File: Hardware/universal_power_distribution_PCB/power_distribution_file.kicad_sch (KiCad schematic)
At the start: 87 parts, among them J1 Screw_Terminal_01x02, J10 Screw_Terminal_01x02, J2 Screw_Terminal_01x02, J3 Screw_Terminal_01x02, J4 Screw_Terminal_01x02, J5 Screw_Terminal_01x02, J6 Screw_Terminal_01x02, J7 Screw_Terminal_01x02, J8 Screw_Terminal_01x02, J9 Screw_Terminal_01x02, Q1 LMR51635XDDCR, Q2 LMR51635XDDCR, Q3 LMR51635XDDCR, Q4 LMR51635XDDCR, Q5 LMR51635XDDCR, Q6 BSS84, U1 INA228, U2 INA228, U3 ACS711xEXLT-31AB

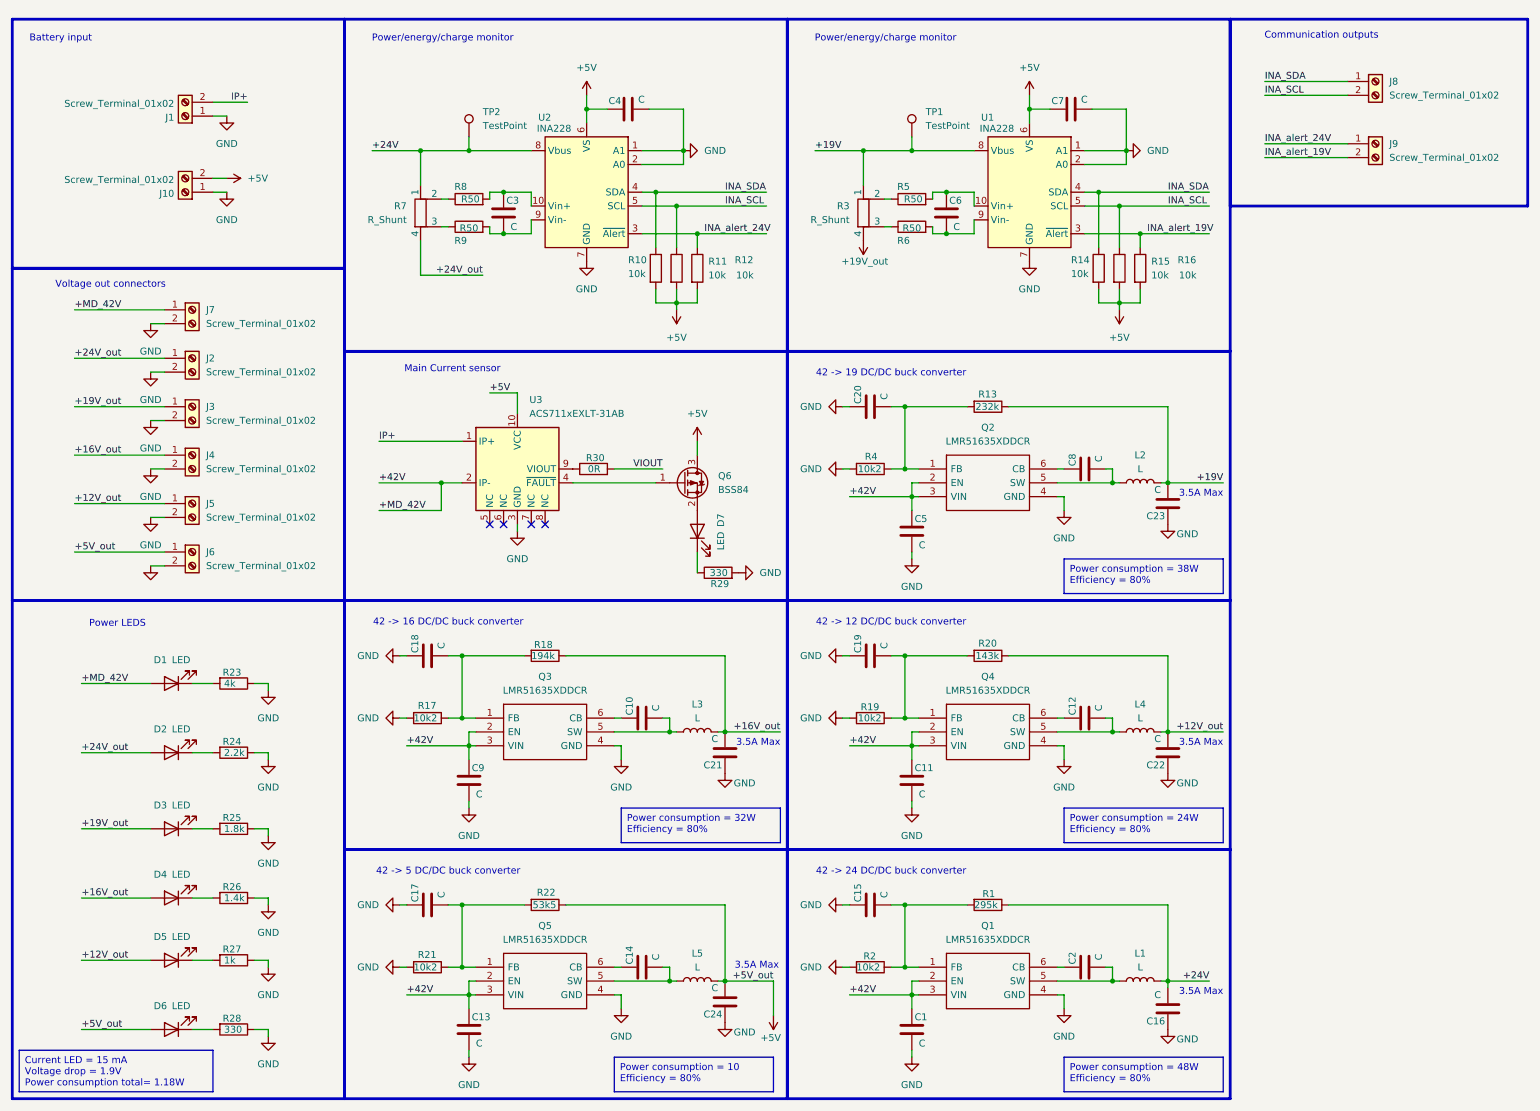
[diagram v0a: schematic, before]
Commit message: Restructured pcb
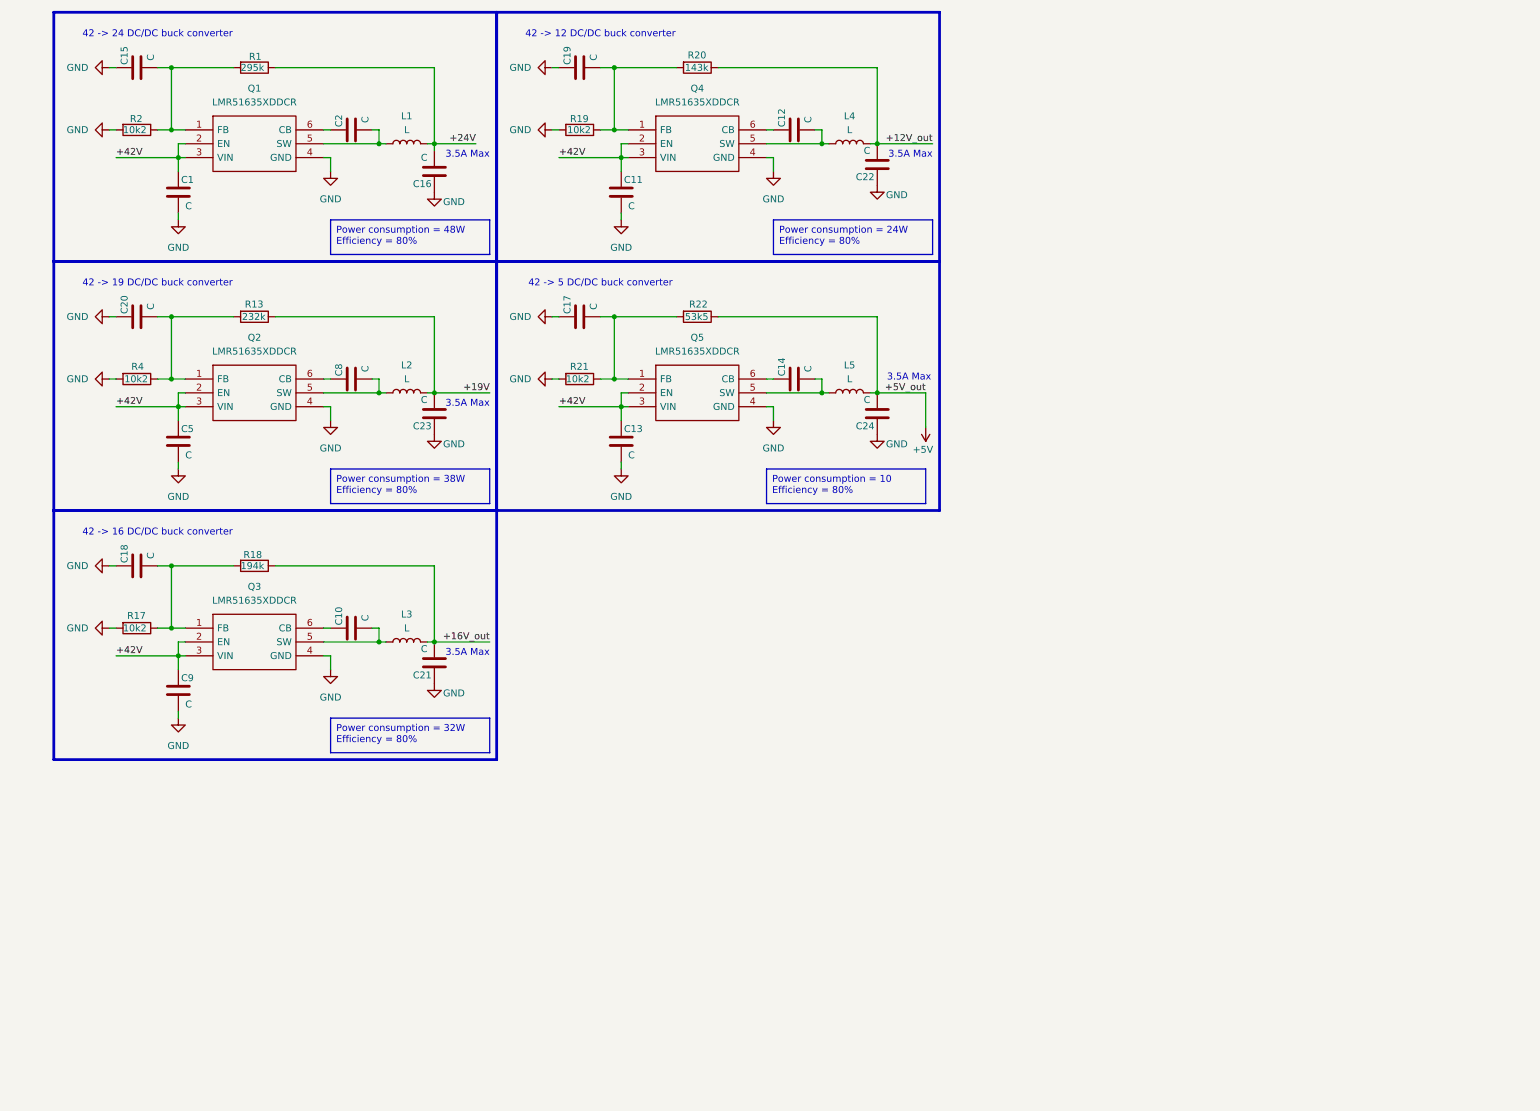
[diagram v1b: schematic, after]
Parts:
- removed C3, C4, C6, C7: C, symbol Device:C
- removed D1, D2, D3, D5, D6: LED, LED_SMD:LED_0603_1608Metric_Pad1.05x0.95mm_HandSolder, symbol Device:LED
- removed D4: LED, Resistor_SMD:R_0603_1608Metric_Pad0.98x0.95mm_HandSolder, symbol Device:LED
- removed D7: LED, symbol Device:LED
- removed J1, J10, J2, J3, J4, J5, J6, J7, J8, J9: Screw_Terminal_01x02, symbol Connector:Screw_Terminal_01x02
- removed Q6: BSS84, Package_TO_SOT_SMD:SOT-23, symbol Transistor_FET:BSS84
- removed R10, R11, R12, R14, R15, R16: 10k, Resistor_SMD:R_0603_1608Metric_Pad0.98x0.95mm_HandSolder, symbol Device:R
- removed R23: 4k, Resistor_SMD:R_0603_1608Metric_Pad0.98x0.95mm_HandSolder, symbol Device:R
- removed R24: 2.2k, Resistor_SMD:R_0603_1608Metric_Pad0.98x0.95mm_HandSolder, symbol Device:R
- removed R25: 1.8k, Resistor_SMD:R_0603_1608Metric_Pad0.98x0.95mm_HandSolder, symbol Device:R
- removed R26: 1.4k, Resistor_SMD:R_0603_1608Metric_Pad0.98x0.95mm_HandSolder, symbol Device:R
- removed R27: 1k, Resistor_SMD:R_0603_1608Metric_Pad0.98x0.95mm_HandSolder, symbol Device:R
- removed R28, R29: 330, Resistor_SMD:R_0603_1608Metric_Pad0.98x0.95mm_HandSolder, symbol Device:R
- removed R3, R7: R_Shunt, symbol Device:R_Shunt
- removed R30: 0R, Resistor_SMD:R_0603_1608Metric_Pad0.98x0.95mm_HandSolder, symbol Device:R
- removed R5, R6, R8, R9: R50, Resistor_SMD:R_0603_1608Metric_Pad0.98x0.95mm_HandSolder, symbol Device:R
- removed TP1, TP2: TestPoint, symbol Connector:TestPoint
- removed U1, U2: INA228, Package_SO:VSSOP-10_3x3mm_P0.5mm, symbol Sensor_Energy:INA228
- removed U3: ACS711xEXLT-31AB, Sensor_Current:Allegro_QFN-12-10-1EP_3x3mm_P0.5mm, symbol Sensor_Current:ACS711xEXLT-31AB
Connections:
- no-connect marks 4 -> 0
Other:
- note removed: "Battery input"
- note removed: "Communication outputs"
- note removed: "Main Current sensor"
- note removed: "Power LEDS"
- note removed: "Power/energy/charge monitor"
- note removed: "Voltage out connectors"
- moved on the sheet: C1, C10, C11, C12, C13, C14, C15, C16, C17, C18, C19, C2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
